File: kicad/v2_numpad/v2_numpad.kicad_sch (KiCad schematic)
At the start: 11 parts, among them J1 Conn_02x08_Top_Bottom

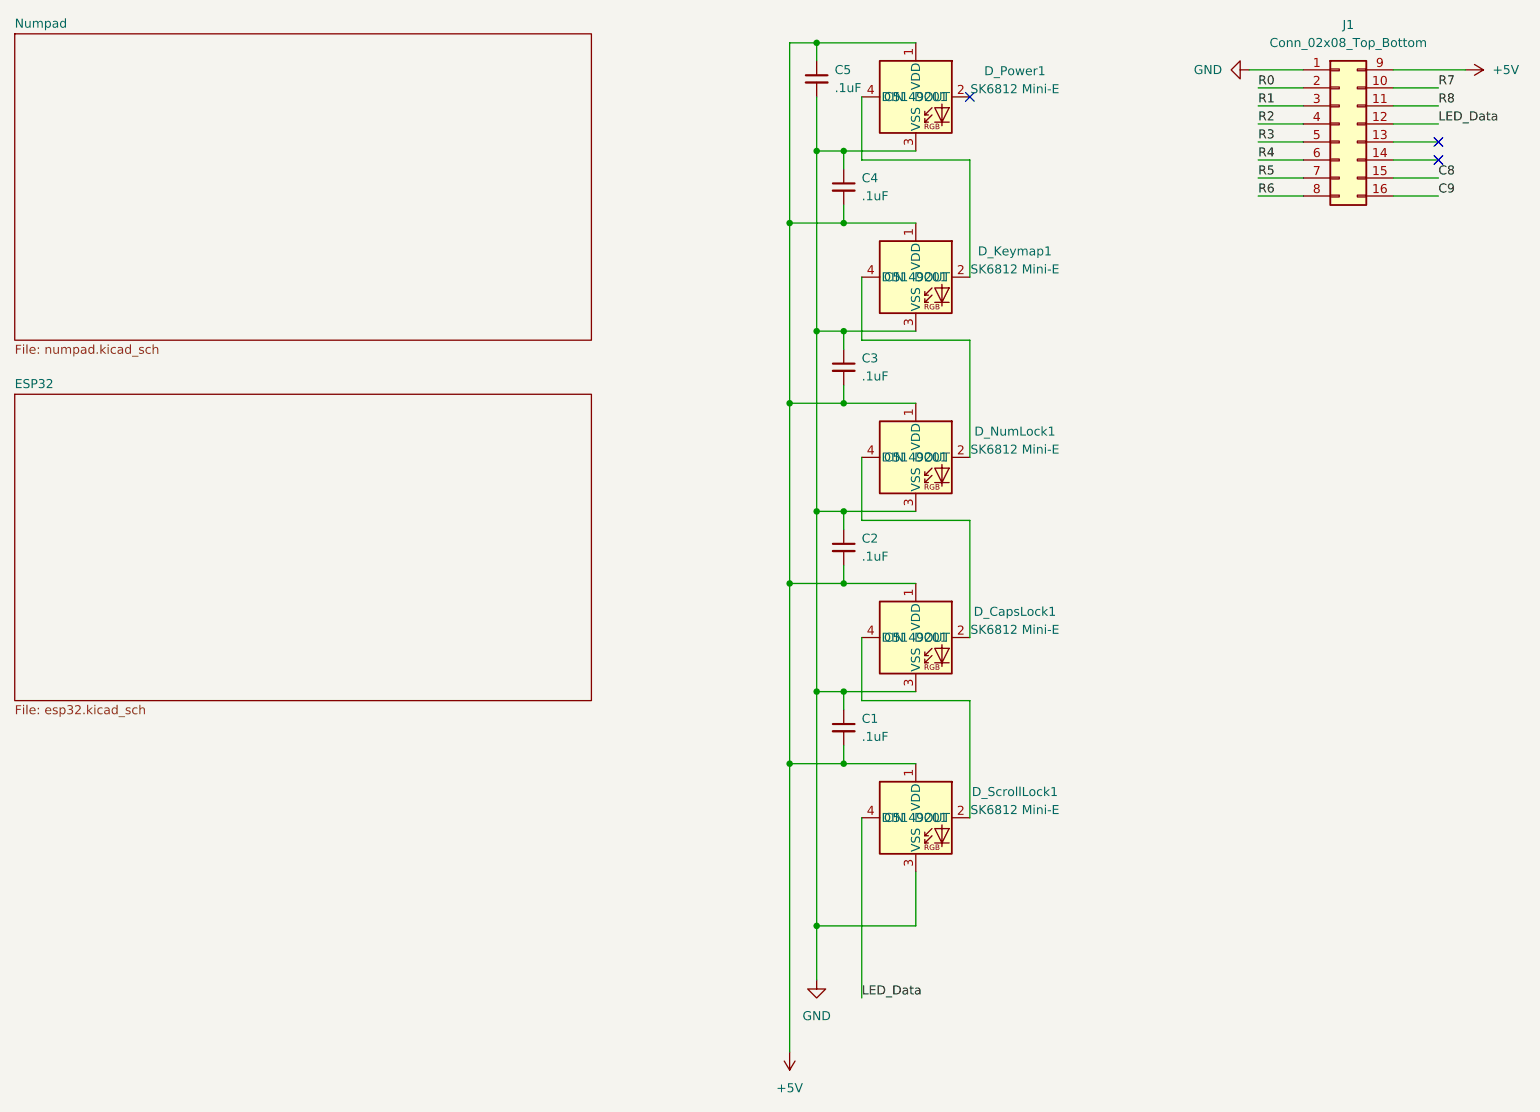
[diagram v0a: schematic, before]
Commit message: [kicad] some more minor tweaks to the numpad
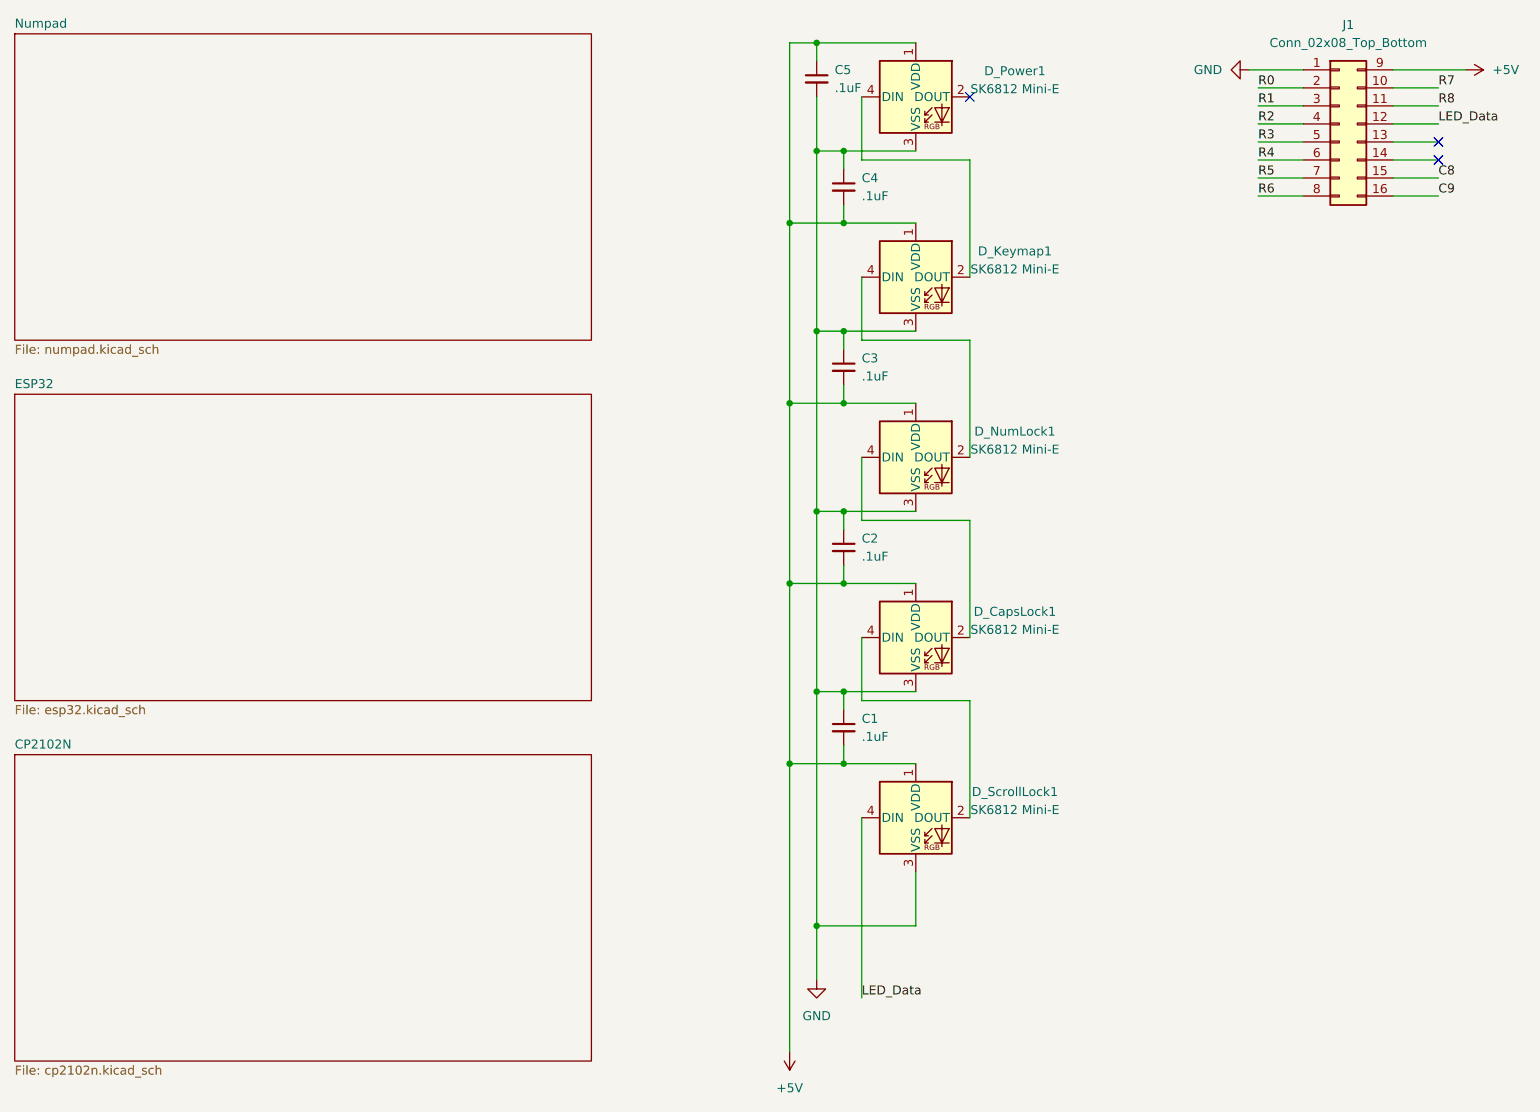
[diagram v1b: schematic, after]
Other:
- added sheet CP2102N (cp2102n.kicad_sch)
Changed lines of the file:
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@@
       (effects (font (size 1.27 1.27)) (justify left top) hide)
     )
-    (property "JLCPCB Part" "C5149201" (at 157.48 139.7 0)
-      (effects (font (size 1.27 1.27)))
+    (property "JLCPCB Part" "C5149201" (at 163.83 153.67 0)
+      (effects (font (size 1.27 1.27)) hide)
     )
     (pin "1")
@@
       (effects (font (size 1.27 1.27)) (justify left top) hide)
     )
-    (property "JLCPCB Part" "C5149201" (at 157.48 38.1 0)
-      (effects (font (size 1.27 1.27)))
+    (property "JLCPCB Part" "C5149201" (at 163.83 52.07 0)
+      (effects (font (size 1.27 1.27)) hide)
     )
     (pin "1")
@@
       (effects (font (size 1.27 1.27)) (justify left top) hide)
     )
-    (property "JLCPCB Part" "C5149201" (at 157.48 114.3 0)
-      (effects (font (size 1.27 1.27)))
+    (property "JLCPCB Part" "C5149201" (at 163.83 128.27 0)
+      (effects (font (size 1.27 1.27)) hide)
     )
     (pin "1")
@@
       (effects (font (size 1.27 1.27)) (justify left top) hide)
     )
-    (property "JLCPCB Part" "C5149201" (at 157.48 88.9 0)
-      (effects (font (size 1.27 1.27)))
+    (property "JLCPCB Part" "C5149201" (at 163.83 102.87 0)
+      (effects (font (size 1.27 1.27)) hide)
     )
     (pin "1")
@@
       (effects (font (size 1.27 1.27)) (justify left top) hide)
     )
-    (property "JLCPCB Part" "C5149201" (at 157.48 63.5 0)
-      (effects (font (size 1.27 1.27)))
+    (property "JLCPCB Part" "C5149201" (at 163.83 77.47 0)
+      (effects (font (size 1.27 1.27)) hide)
     )
     (pin "1")
@@
       )
     )
+  )
+  (sheet (at 30.48 130.81) (size 81.28 43.18) (fields_autoplaced)
+    (stroke (width 0.1524) (type solid))
+    (fill (color 0 0 0 0.0000))
+    (property "Sheetname" "CP2102N" (at 30.48 130.0984 0)
+      (effects (font (size 1.27 1.27)) (justify left bottom))
+    )
+    (property "Sheetfile" "cp2102n.kicad_sch" (at 30.48 174.5746 0)
+      (effects (font (size 1.27 1.27)) (justify left top))
+    )
+    (instances
+      (project "v2_numpad"
+        (path "/42eee74c-d04d-4a1d-8e02-a7aca1694734" (page "4"))
+      )
+    )
